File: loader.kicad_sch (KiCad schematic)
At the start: 6 parts, among them J2 LOADER_CONSOLE, J3 SPI, J5 68K_CONSOLE, U2 FT232RL, U3 ATmega2560-16A, U7 W25Q128JVS

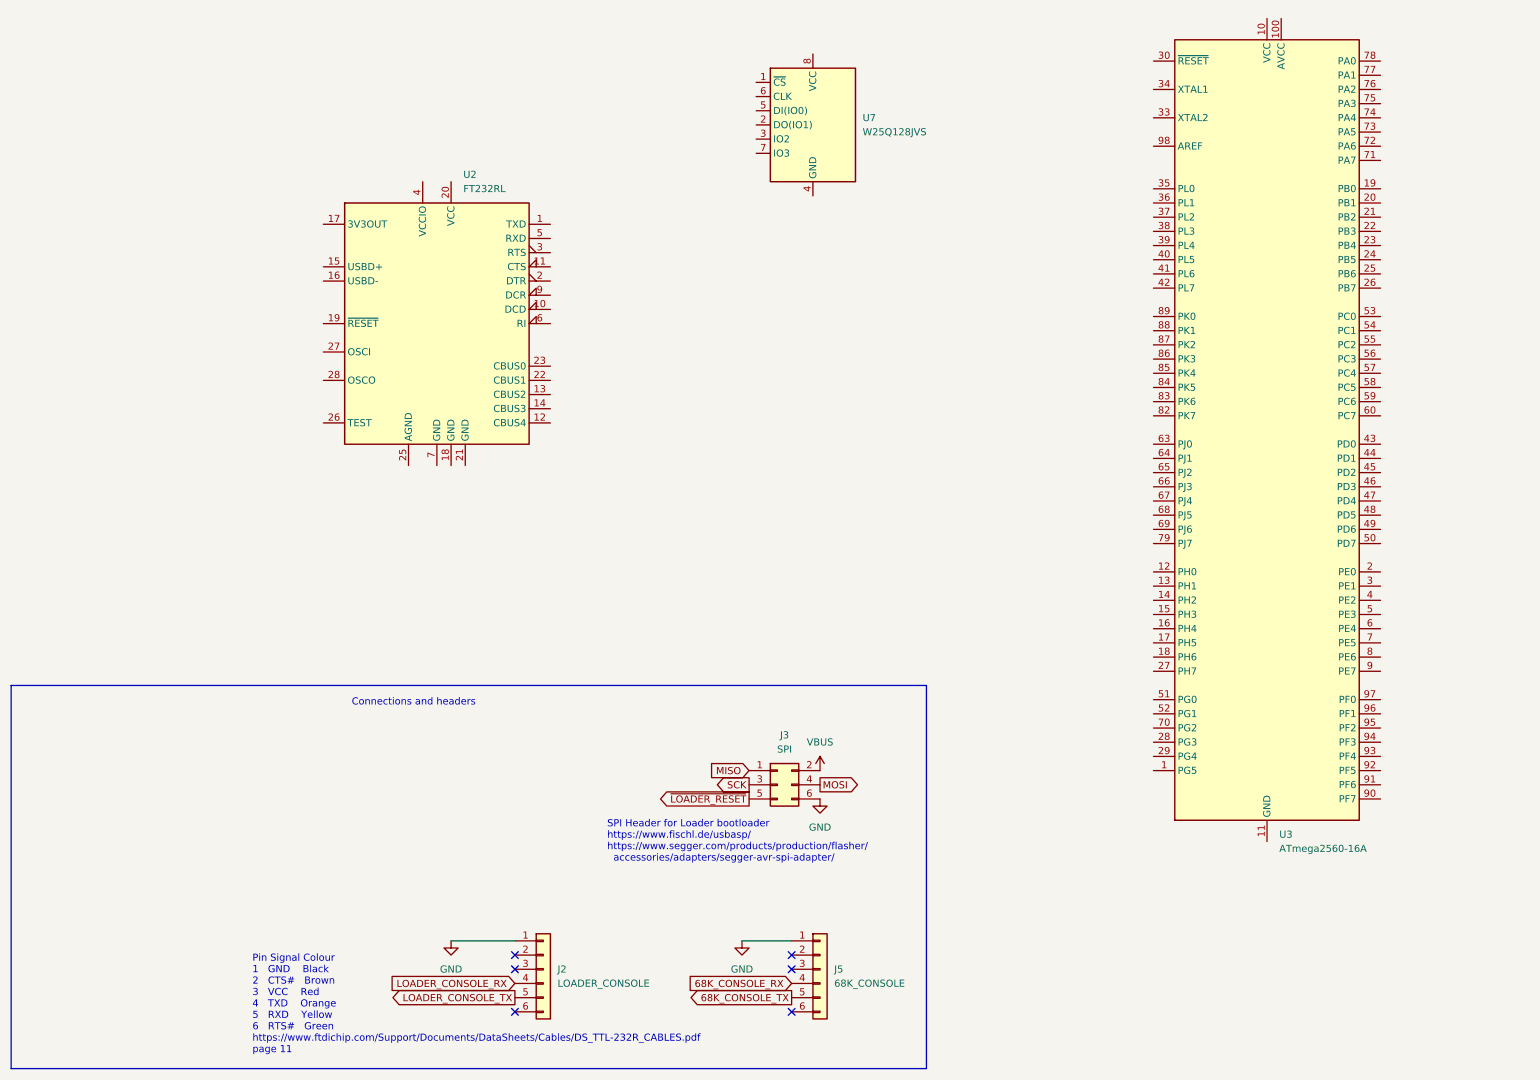
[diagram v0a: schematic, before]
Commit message: updates
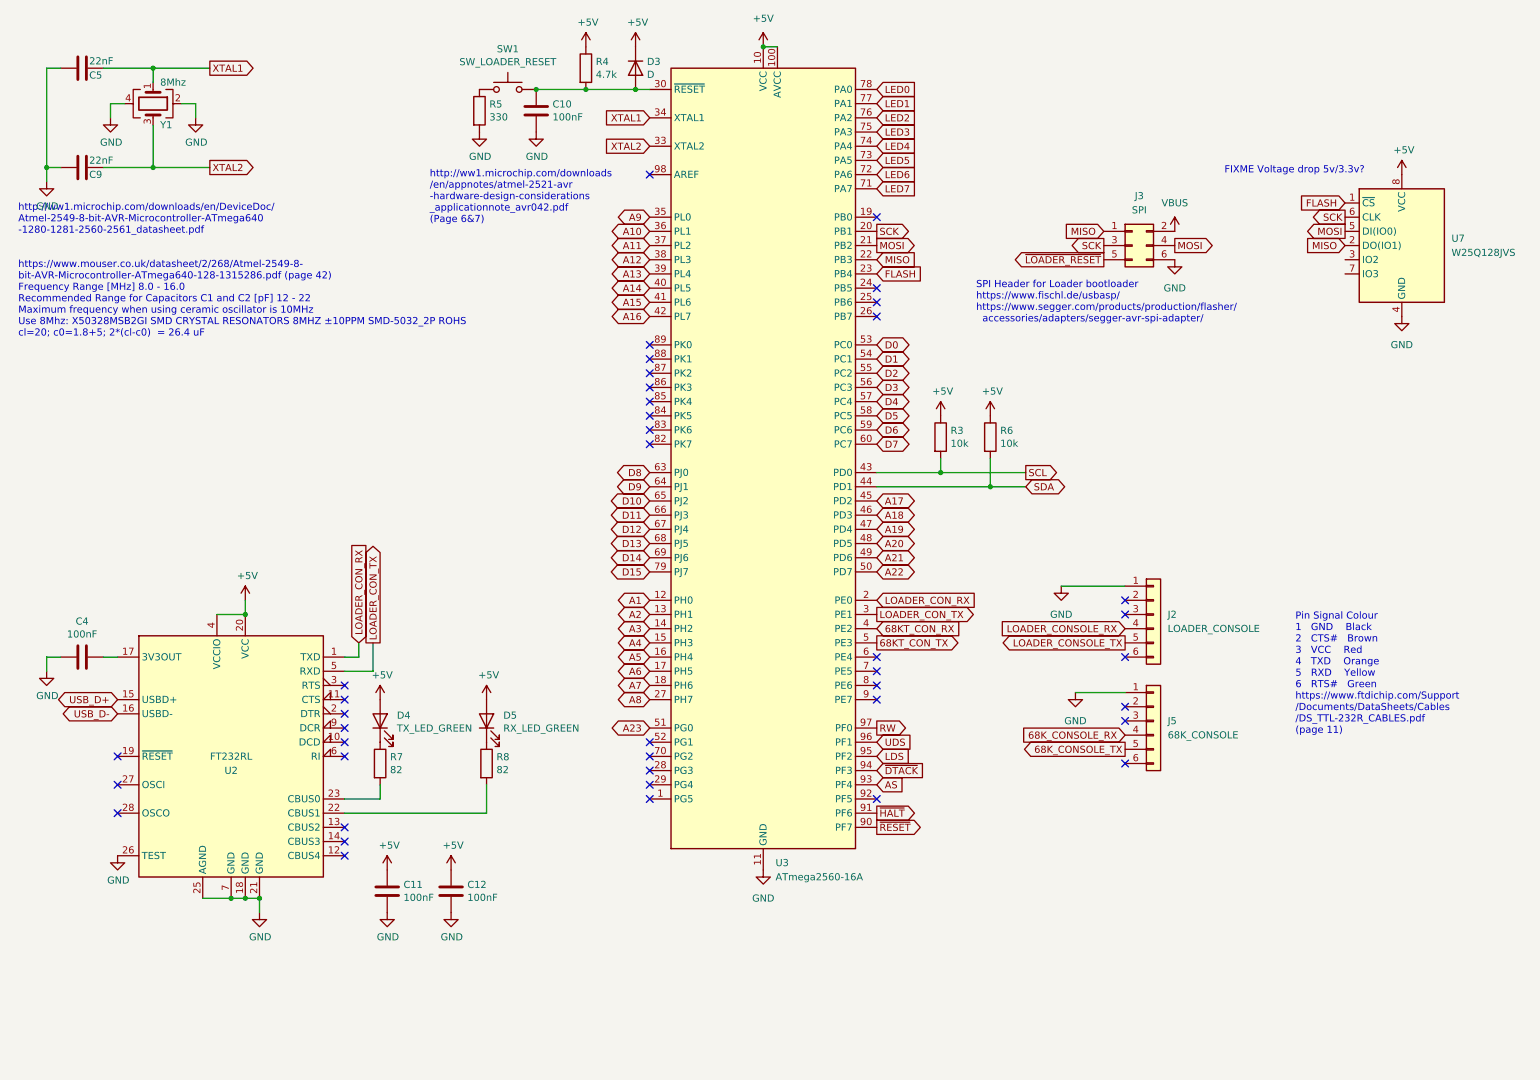
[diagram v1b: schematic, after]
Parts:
- added C10, C11, C12, C4: 100nF, Capacitor_SMD:C_0603_1608Metric, symbol Device:C
- added C5, C9: 22nF, Capacitor_SMD:C_0603_1608Metric, symbol Device:C
- added D3: D, Diode_SMD:D_SMA, symbol Device:D
- added D4: TX_LED_GREEN, LED_SMD:LED_0603_1608Metric, symbol Device:LED
- added D5: RX_LED_GREEN, LED_SMD:LED_0603_1608Metric, symbol Device:LED
- added R3, R6: 10k, Resistor_SMD:R_0603_1608Metric, symbol Device:R
- added R4: 4.7k, Resistor_SMD:R_0603_1608Metric, symbol Device:R
- added R5: 330, Resistor_SMD:R_0603_1608Metric, symbol Device:R
- added R7, R8: 82, Resistor_SMD:R_0603_1608Metric, symbol Device:R
- added SW1: SW_LOADER_RESET, Button_Switch_SMD:SW_Push_1P1T_XKB_TS-1187A, symbol Switch:SW_Push
- added Y1: 8Mhz, Crystal:Crystal_SMD_5032-4Pin_5.0x3.2mm, symbol Device:Crystal_GND24
- U2: JLPCB Datasheet (none) -> https://datasheet.lcsc.com/szlcsc/Future-Designs-FT232RL-RE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; JLPCB Part C8690 -> FT232RL-REEL
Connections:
- net GND: now also U2.18 (GND), U2.21 (GND), U2.25 (AGND), U2.26 (TEST), U2.7 (GND), U3.11 (GND), U3.32 (GND), U3.62 (GND), U3.81 (GND), U3.99 (GND), U7.4 (GND), C10.2, C11.2, C12.2, C4.2, C5.1, C9.1, R5.2, Y1.2, Y1.4
- net MISO: now also U3.22 (PB3), U7.2 (DO(IO1))
- net MOSI: now also U3.21 (PB2), U7.5 (DI(IO0))
- net SCK: now also U3.20 (PB1), U7.6 (CLK)
- net FLASH: now reaches U7.1 (~{CS})
- net FLASH: now also U3.23 (PB4)
- net +5V: now reaches U7.8 (VCC)
- net +5V: now also U2.20 (VCC), U2.4 (VCCIO), U3.10 (VCC), U3.100 (AVCC), U3.31 (VCC), U3.61 (VCC), U3.80 (VCC), C11.1, C12.1, D3.1 (K), D4.2 (A), D5.2 (A), R3.1, R4.1, R6.1
- net A1: now reaches U3.12 (PH0)
- net A2: now reaches U3.13 (PH1)
- net A3: now reaches U3.14 (PH2)
- net A4: now reaches U3.15 (PH3)
- net A5: now reaches U3.16 (PH4)
- net A6: now reaches U3.17 (PH5)
- net A7: now reaches U3.18 (PH6)
- net LOADER_CON_RX: now reaches U3.2 (PE0)
- net LOADER_CON_RX: now also U2.1 (TXD)
- net A8: now reaches U3.27 (PH7)
- net LOADER_CON_TX: now reaches U3.3 (PE1)
- net LOADER_CON_TX: now also U2.5 (RXD)
- net at U3.30 (~{RESET}): now also C10.1, D3.2 (A), R4.2, SW1.2
- net XTAL2: now reaches U3.33 (XTAL2)
- net XTAL2: now also C9.2, Y1.3
- net XTAL1: now reaches U3.34 (XTAL1)
- net XTAL1: now also C5.2, Y1.1
- net A9: now reaches U3.35 (PL0)
- net A10: now reaches U3.36 (PL1)
- net A11: now reaches U3.37 (PL2)
- net A12: now reaches U3.38 (PL3)
- net A13: now reaches U3.39 (PL4)
- net 68KT_CON_RX: now reaches U3.4 (PE2)
- net A14: now reaches U3.40 (PL5)
- net A15: now reaches U3.41 (PL6)
- net A16: now reaches U3.42 (PL7)
- net SCL: now reaches U3.43 (PD0)
- net SCL: now also R3.2
- net SDA: now reaches U3.44 (PD1)
- net SDA: now also R6.2
- net A17: now reaches U3.45 (PD2)
- net A18: now reaches U3.46 (PD3)
- net A19: now reaches U3.47 (PD4)
- net A20: now reaches U3.48 (PD5)
- net A21: now reaches U3.49 (PD6)
- net 68KT_CON_TX: now reaches U3.5 (PE3)
- net A22: now reaches U3.50 (PD7)
- net A23: now reaches U3.51 (PG0)
- net D0: now reaches U3.53 (PC0)
- net D1: now reaches U3.54 (PC1)
- net D2: now reaches U3.55 (PC2)
- net D3: now reaches U3.56 (PC3)
- net D4: now reaches U3.57 (PC4)
- net D5: now reaches U3.58 (PC5)
- net D6: now reaches U3.59 (PC6)
- net D7: now reaches U3.60 (PC7)
- net D8: now reaches U3.63 (PJ0)
- net D9: now reaches U3.64 (PJ1)
- net D10: now reaches U3.65 (PJ2)
- net D11: now reaches U3.66 (PJ3)
- net D12: now reaches U3.67 (PJ4)
- net D13: now reaches U3.68 (PJ5)
- net D14: now reaches U3.69 (PJ6)
- net LED7: now reaches U3.71 (PA7)
- net LED6: now reaches U3.72 (PA6)
- net LED5: now reaches U3.73 (PA5)
- net LED4: now reaches U3.74 (PA4)
- net LED3: now reaches U3.75 (PA3)
- net LED2: now reaches U3.76 (PA2)
- net LED1: now reaches U3.77 (PA1)
- net LED0: now reaches U3.78 (PA0)
- net D15: now reaches U3.79 (PJ7)
- net ~{RESET}: now reaches U3.90 (PF7)
- net ~{HALT}: now reaches U3.91 (PF6)
- net AS: now reaches U3.93 (PF4)
- net ~{DTACK}: now reaches U3.94 (PF3)
- net LDS: now reaches U3.95 (PF2)
- net UDS: now reaches U3.96 (PF1)
- net RW: now reaches U3.97 (PF0)
- net USB_D+: now reaches U2.15 (USBD+)
- net USB_D-: now reaches U2.16 (USBD-)
- net at U2.17 (3V3OUT): now also C4.1
- net at U2.22 (CBUS1): now also R8.2
- net at U2.23 (CBUS0): now also R7.2
- new net: D4.1 (K), R7.1
- new net: D5.1 (K), R8.1
- new net: R5.1, SW1.1
- no-connect marks 6 -> 41
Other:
- note added: "FIXME Voltage drop 5v/3.3v?"
- note added: "Pin Signal Colour 1 GND Black 2 CTS# Brown 3 VCC Red 4 TXD Orange 5 RXD Yellow 6 RTS# Green https://www.ftdichip.com/Support /Documents/DataSheets/Cables /DS_TTL-232R_CABLES.pdf (page 11)"
- note added: "http://ww1.microchip.com/downloads /en/appnotes/atmel-2521-avr -hardware-design-considerations _applicationnote_avr042.pdf (Page 6&7)"
- note added: "http://ww1.microchip.com/downloads/en/DeviceDoc/ Atmel-2549-8-bit-AVR-Microcontroller-ATmega640 -1280-1281-2560-2561_datasheet.pdf https://www.mouser.co.uk/datasheet/2/268/Atmel-2549-8- bit-AVR-Microcontroller-ATmega640-128-1315286.pdf (page 42) Frequency Range [MHz] 8.0 - 16.0 Recommended Range for Capacitors C1 and C2 [pF] 12 - 22 Maximum frequency when using ceramic oscillator is 10MHz Use 8Mh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"
- note removed: "Connections and headers"
- note removed: "Pin Signal Colour 1 GND Black 2 CTS# Brown 3 VCC Red 4 TXD Orange 5 RXD Yellow 6 RTS# Green https://www.ftdichip.com/Support/Documents/DataSheets/Cables/DS_TTL-232R_CABLES.pdf page 11"
- moved on the sheet: J2, J3, J5, U3, U7
